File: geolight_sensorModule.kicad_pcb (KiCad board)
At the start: 2 copper layers, 19 parts, among them IC1 ATTINY841, P1 5V, P2 ICSP, P3 IN, P4 OUT, P5 AUX_SENSOR, P6 UART, U1 TCRT5000/L, Y1 16Mhz

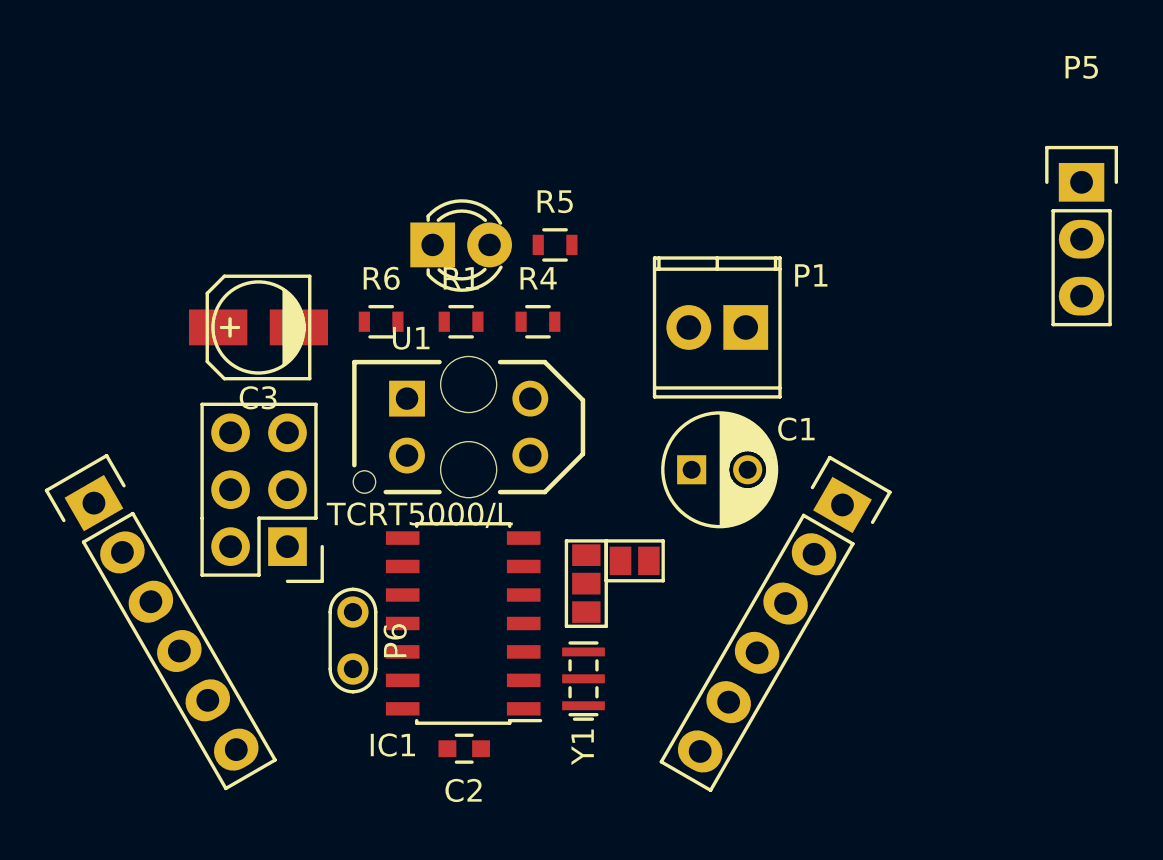
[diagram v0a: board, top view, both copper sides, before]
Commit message: re-arranged PCB, routing done (all except ground plane)
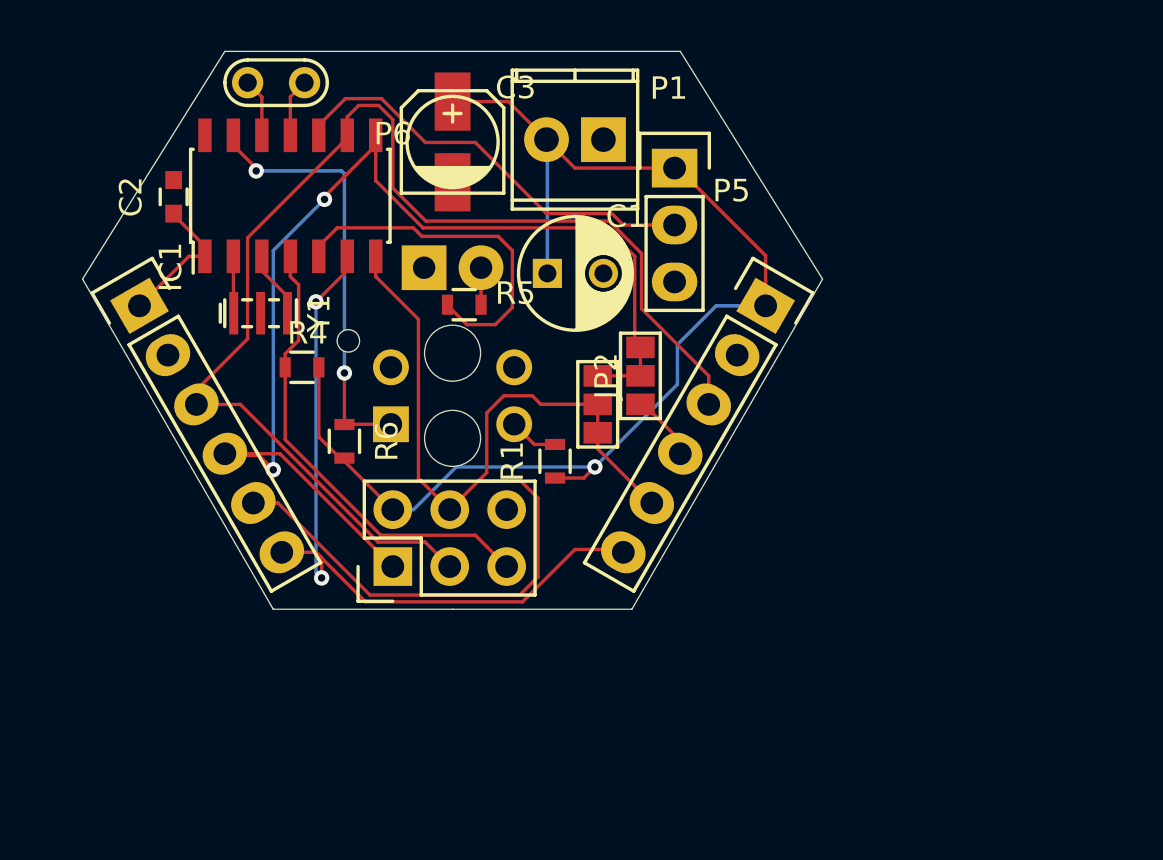
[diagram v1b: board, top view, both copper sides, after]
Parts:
- D1, U1: moved to B.Cu
- IC1: value ATTINY841 -> ATTINY841-SSU
- JP2: footprint Connect:GS2 -> Connect:GS3
- moved C2 27.8 mm to (145.0, 114.9), turned to 90 degrees
- moved P6 25.1 mm to (149.6, 109.9), turned to 180 degrees
- moved Y1 21.8 mm to (148.9, 120.1), turned to 0 degrees
- moved IC1 20.6 mm to (150.2, 114.9), turned to 90 degrees
- moved P5 18.2 mm to (167.4, 113.7)
- moved C3 12.0 mm to (157.5, 112.5), turned to 90 degrees
- moved C1 10.9 mm to (161.7, 118.4)
- moved R4 10.7 mm to (150.8, 122.6), turned to 180 degrees
- moved P1 10.5 mm to (164.2, 112.4)
- moved P4 9.52 mm to (171.4, 119.8)
- moved P3 9.04 mm to (143.5, 119.8)
- moved JP2 8.26 mm to (165.9, 122.9), turned to 180 degrees
- moved JP1 8.02 mm to (164.0, 124.2)
- moved R1 7.50 mm to (162.1, 126.7), turned to 90 degrees
- moved R6 5.58 mm to (152.7, 125.9), turned to 270 degrees
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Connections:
- IC1 pad 4: Net-(IC1-Pad4) -> /RESET
- R4 pad 2: Net-(IC1-Pad4) -> /RESET
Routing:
- net +5V: track 0.00 -> 62.6 mm, vias 0 -> 1
- net /SCK/SCL: track 0.00 -> 55.8 mm
- net /MISO: track 0.00 -> 50.5 mm, vias 0 -> 2
- net /SDA/MOSI: track 0.00 -> 49.7 mm
- net /SS: track 0.00 -> 33.5 mm, vias 0 -> 2
- net /RESET: track 0.00 -> 20.8 mm
- net Net-(IC1-Pad13): track 0.00 -> 19.3 mm, vias 0 -> 2
- net /AUX: track 0.00 -> 19.2 mm
- net Net-(IC1-Pad5): track 0.00 -> 16.0 mm
- net Net-(JP2-Pad1): track 0.00 -> 3.03 mm
- net Net-(IC1-Pad3): track 0.00 -> 3.01 mm
- net /TX: track 0.00 -> 2.61 mm
- net /RX: track 0.00 -> 2.61 mm
- net Net-(IC1-Pad2): track 0.00 -> 2.55 mm
- net Net-(R1-Pad2): track 0.00 -> 2.20 mm
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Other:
- board outline added: 33 x 24.9 mm

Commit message: finished v0.99 (no top copper pour)
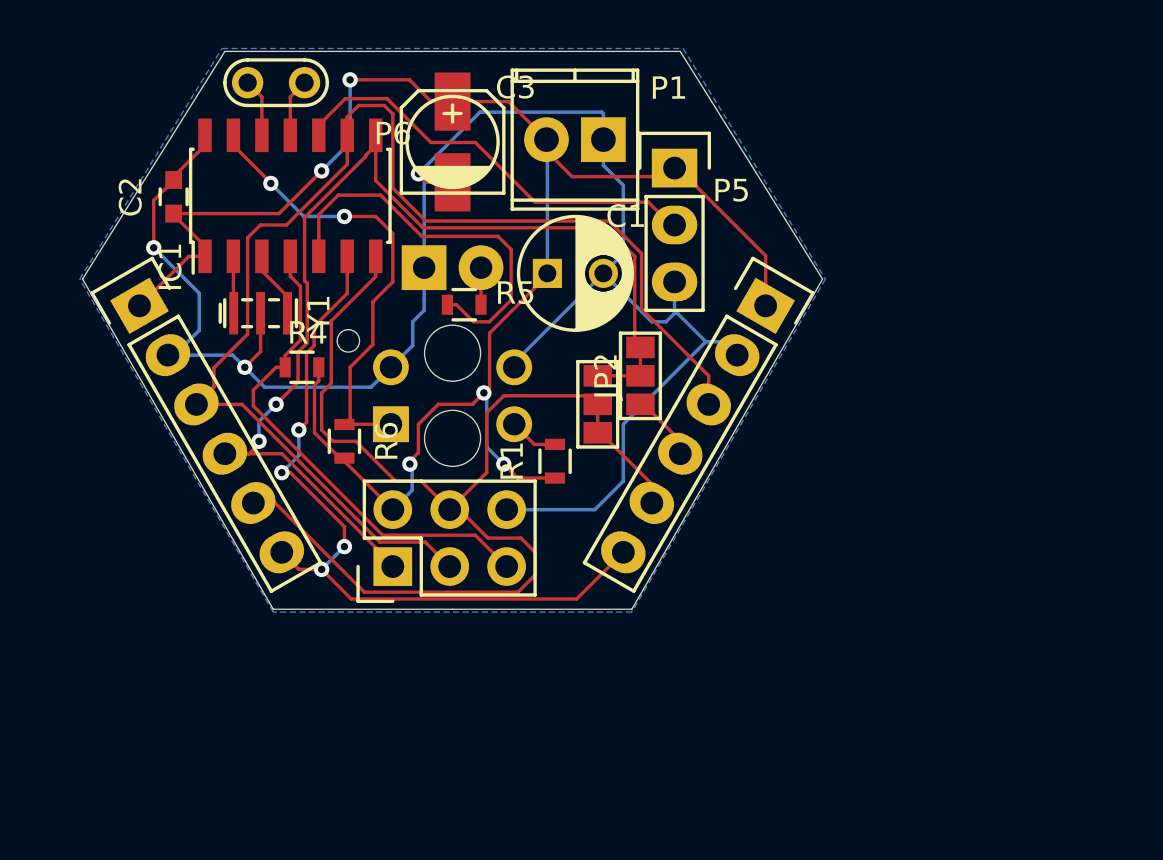
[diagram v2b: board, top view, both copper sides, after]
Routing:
- net GND: track 0.00 -> 82.8 mm, vias 0 -> 3
- net +5V: track 62.6 -> 77.4 mm, vias 1 -> 5
- net /SDA/MOSI: track 49.7 -> 52.1 mm
- net Net-(IC1-Pad5): track 16.0 -> 17.6 mm
- net Net-(IC1-Pad13): track 19.3 -> 20.7 mm
- net /RESET: track 20.8 -> 22.2 mm
- net /SCK/SCL: track 55.8 -> 56.6 mm
- net /MISO: track 50.5 -> 49.7 mm
- net /SS: track 33.5 -> 33.9 mm, vias 2 -> 4
- added copper zone on B.Cu, net GND
